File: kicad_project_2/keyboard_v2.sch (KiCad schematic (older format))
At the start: 170 parts, among them SW1 SW_Push, U1 ATMEGA32U4, Y1 16MHz

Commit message: fix pcb
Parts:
- C1, C2: footprint kbd:D3_TH_SMD -> kbd:D3_SMD_v2
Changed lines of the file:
@@
 F 0 "C1" V 5671 8400 50  0000 C CNN
 F 1 "22pF" V 5762 8400 50  0000 C CNN
-F 2 "kbd:D3_TH_SMD" H 5900 8400 50  0001 C CNN
+F 2 "kbd:D3_SMD_v2" H 5900 8400 50  0001 C CNN
 F 3 "~" H 5900 8400 50  0001 C CNN
 	1    5900 8400
@@
 F 0 "C2" V 5671 8650 50  0000 C CNN
 F 1 "22pF" V 5762 8650 50  0000 C CNN
-F 2 "kbd:D3_TH_SMD" H 5900 8650 50  0001 C CNN
+F 2 "kbd:D3_SMD_v2" H 5900 8650 50  0001 C CNN
 F 3 "~" H 5900 8650 50  0001 C CNN
 	1    5900 8650

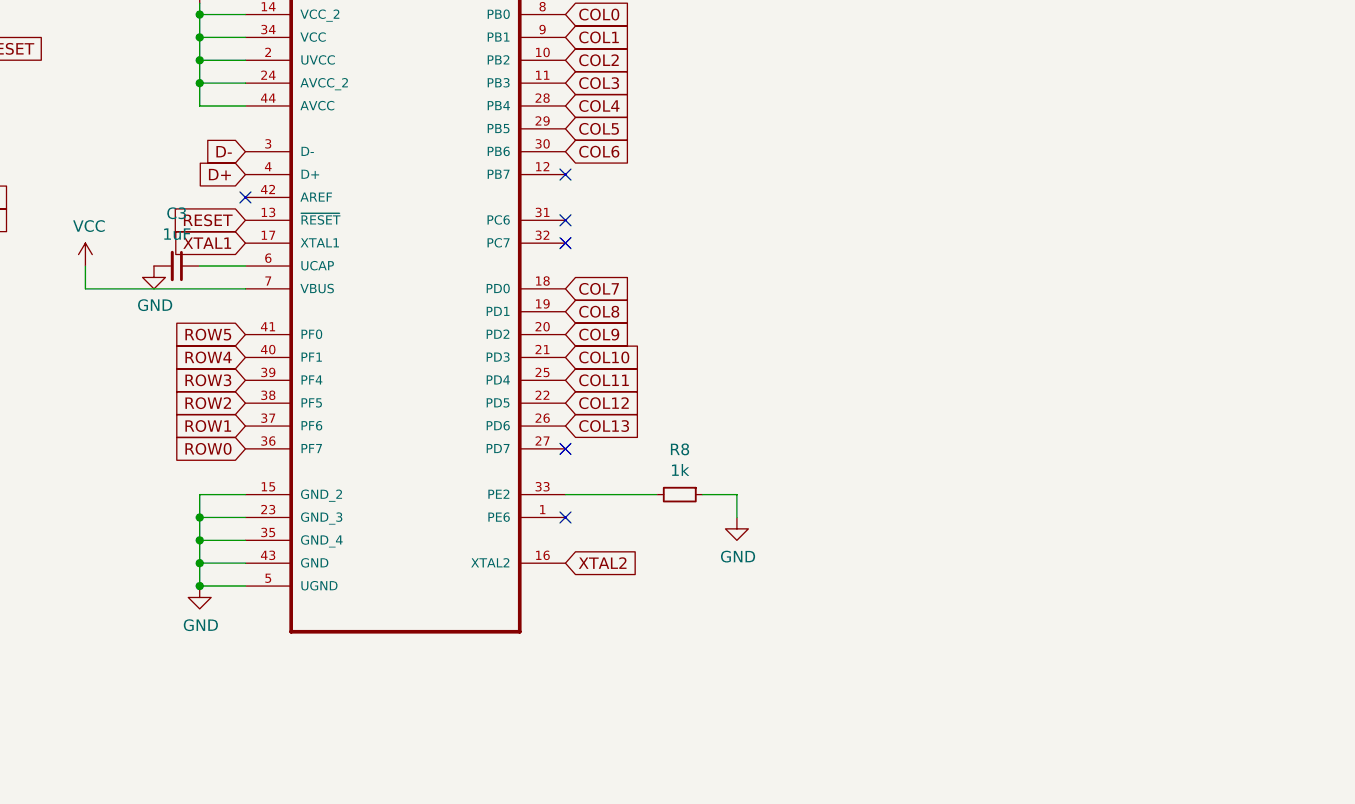
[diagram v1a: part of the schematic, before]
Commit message: fix pcb
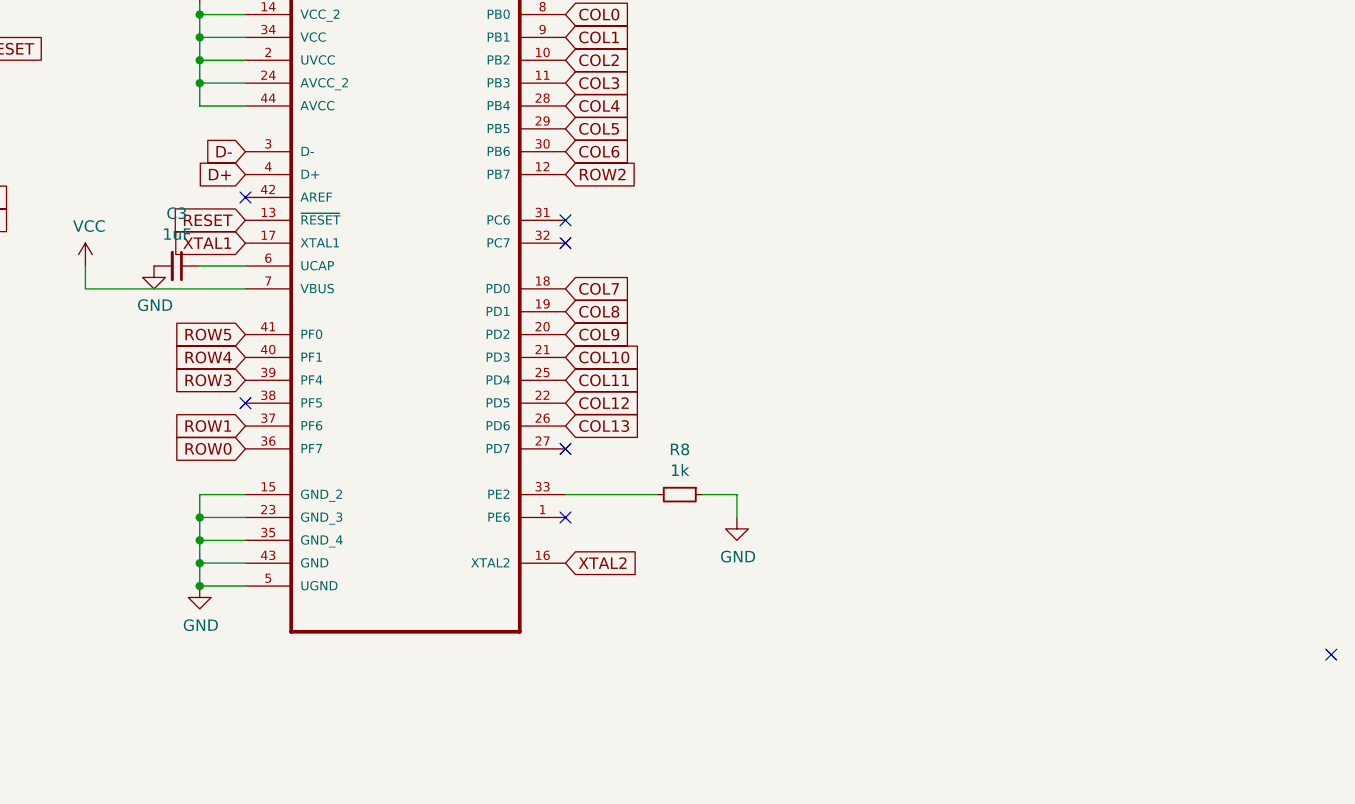
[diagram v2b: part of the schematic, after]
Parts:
- F1, F2, MX1, MX10, MX11, MX12, MX13, MX14, MX15, MX16, MX17, MX18, MX19, MX2, MX20, MX21, MX22, MX23, MX24, MX25, MX26, MX27, MX28, MX29, MX3, MX30, MX31, MX32, MX33, MX34, MX35, MX36, MX37, MX38, MX39, MX4, MX40, MX41, MX42, MX43, MX44, MX45, MX46, MX47, MX48, MX49, MX5, MX50, MX51, MX52, MX53, MX54, MX55, MX56, MX57, MX58, MX59, MX6, MX60, MX61, MX62, MX63, MX64, MX65, MX66, MX67, MX68, MX69, MX7, MX70, MX8, MX9: footprint MX_Alps_Hybrid:MX-1U-NoLED -> Alps_Only:ALPS-1U
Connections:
- net ROW2: now also U1.12 (PB7); no longer U1.38 (PF5)
- no-connect marks 10 -> 11

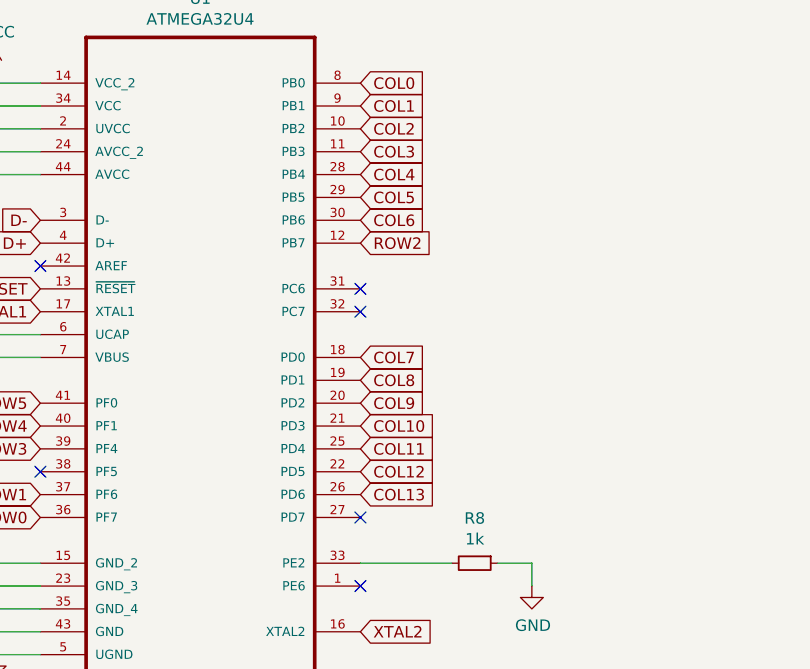
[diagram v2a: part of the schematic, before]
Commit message: fix pcb
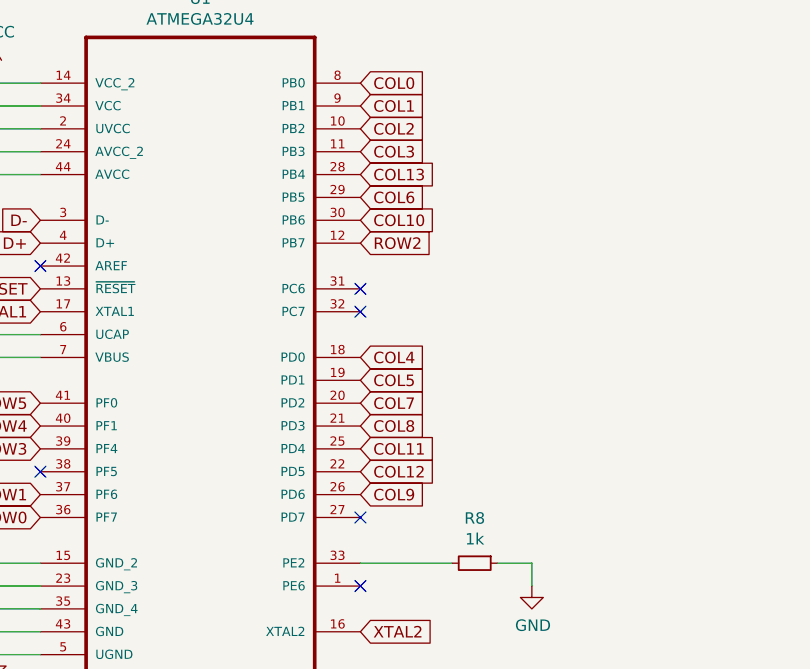
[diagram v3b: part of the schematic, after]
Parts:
- C1, C2: footprint kbd:D3_SMD_v2 -> kbd:D3_TH_SMD
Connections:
- net COL10: now also U1.30 (PB6); no longer U1.21 (PD3)
- net COL13: now also U1.28 (PB4); no longer U1.26 (PD6)
- net COL4: now also U1.18 (PD0); no longer U1.28 (PB4)
- net COL5: now also U1.19 (PD1); no longer U1.29 (PB5)
- net COL6: now also U1.29 (PB5); no longer U1.30 (PB6)
- net COL7: now also U1.20 (PD2); no longer U1.18 (PD0)
- net COL8: now also U1.21 (PD3); no longer U1.19 (PD1)
- net COL9: now also U1.26 (PD6); no longer U1.20 (PD2)
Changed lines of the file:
@@
 F 0 "C1" V 5671 8400 50  0000 C CNN
 F 1 "22pF" V 5762 8400 50  0000 C CNN
-F 2 "kbd:D3_SMD_v2" H 5900 8400 50  0001 C CNN
+F 2 "kbd:D3_TH_SMD" H 5900 8400 50  0001 C CNN
 F 3 "~" H 5900 8400 50  0001 C CNN
 	1    5900 8400
@@
 F 0 "C2" V 5671 8650 50  0000 C CNN
 F 1 "22pF" V 5762 8650 50  0000 C CNN
-F 2 "kbd:D3_SMD_v2" H 5900 8650 50  0001 C CNN
+F 2 "kbd:D3_TH_SMD" H 5900 8650 50  0001 C CNN
 F 3 "~" H 5900 8650 50  0001 C CNN
 	1    5900 8650
@@
 	6000 10400 6250 10400
 Connection ~ 6250 10400
-Text GLabel 9700 8050 2    50   Input ~ 0
-COL4
-Text GLabel 9700 8150 2    50   Input ~ 0
-COL5
-Text GLabel 9700 8250 2    50   Input ~ 0
-COL6
-Text GLabel 9700 8850 2    50   Input ~ 0
+Text GLabel 9700 9050 2    50   Input ~ 0
 COL7
-Text GLabel 9700 8950 2    50   Input ~ 0
-COL8
-Text GLabel 9700 9050 2    50   Input ~ 0
+Text GLabel 9700 9450 2    50   Input ~ 0
 COL9
-Text GLabel 9700 9150 2    50   Input ~ 0
-COL10
-Text GLabel 9700 9250 2    50   Input ~ 0
-COL11
 $Comp
 L power:PWR_FLAG #FLG01
@@
 Wire Wire Line
 	9150 850  9150 1650
-Text GLabel 9700 9350 2    50   Input ~ 0
-COL12
-Text GLabel 9700 9450 2    50   Input ~ 0
-COL13
 Text GLabel 750  4500 0    50   Input ~ 0
 ROW5
@@
 NoConn ~ 8300 9350
 NoConn ~ 13050 10450
+Text GLabel 9700 8950 2    50   Input ~ 0
+COL5
+Text GLabel 9700 8850 2    50   Input ~ 0
+COL4
+Text GLabel 9700 9350 2    50   Input ~ 0
+COL12
+Text GLabel 9700 9250 2    50   Input ~ 0
+COL11
+Text GLabel 9700 8250 2    50   Input ~ 0
+COL10
+Text GLabel 9700 8150 2    50   Input ~ 0
+COL6
+Text GLabel 9700 8050 2    50   Input ~ 0
+COL13
+Text GLabel 9700 9150 2    50   Input ~ 0
+COL8
 $EndSCHEMATC

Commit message: add dxf
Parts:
- C1, C2: footprint kbd:D3_TH_SMD -> Capacitor_SMD:C_1206_3216Metric_Pad1.42x1.75mm_HandSolder
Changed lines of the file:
@@
 F 0 "C1" V 5671 8400 50  0000 C CNN
 F 1 "22pF" V 5762 8400 50  0000 C CNN
-F 2 "kbd:D3_TH_SMD" H 5900 8400 50  0001 C CNN
+F 2 "Capacitor_SMD:C_1206_3216Metric_Pad1.42x1.75mm_HandSolder" H 5900 8400 50  0001 C CNN
 F 3 "~" H 5900 8400 50  0001 C CNN
 	1    5900 8400
@@
 F 0 "C2" V 5671 8650 50  0000 C CNN
 F 1 "22pF" V 5762 8650 50  0000 C CNN
-F 2 "kbd:D3_TH_SMD" H 5900 8650 50  0001 C CNN
+F 2 "Capacitor_SMD:C_1206_3216Metric_Pad1.42x1.75mm_HandSolder" H 5900 8650 50  0001 C CNN
 F 3 "~" H 5900 8650 50  0001 C CNN
 	1    5900 8650
